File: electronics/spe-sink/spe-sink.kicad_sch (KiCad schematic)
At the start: 14 parts, among them J1 CONN_01X05_RA

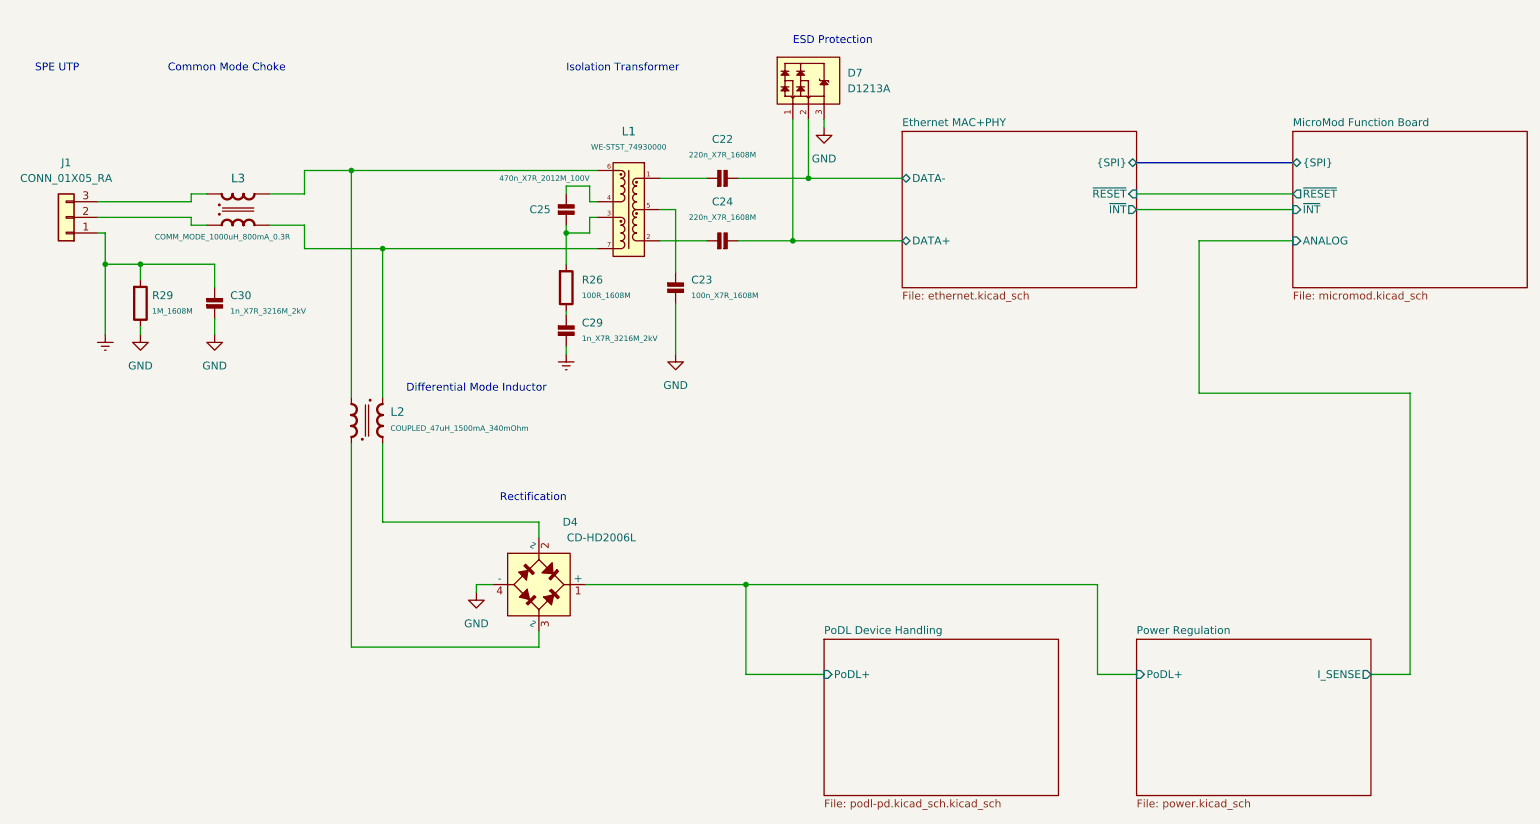
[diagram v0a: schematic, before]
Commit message: Random uncommitted KiCAD tweaks
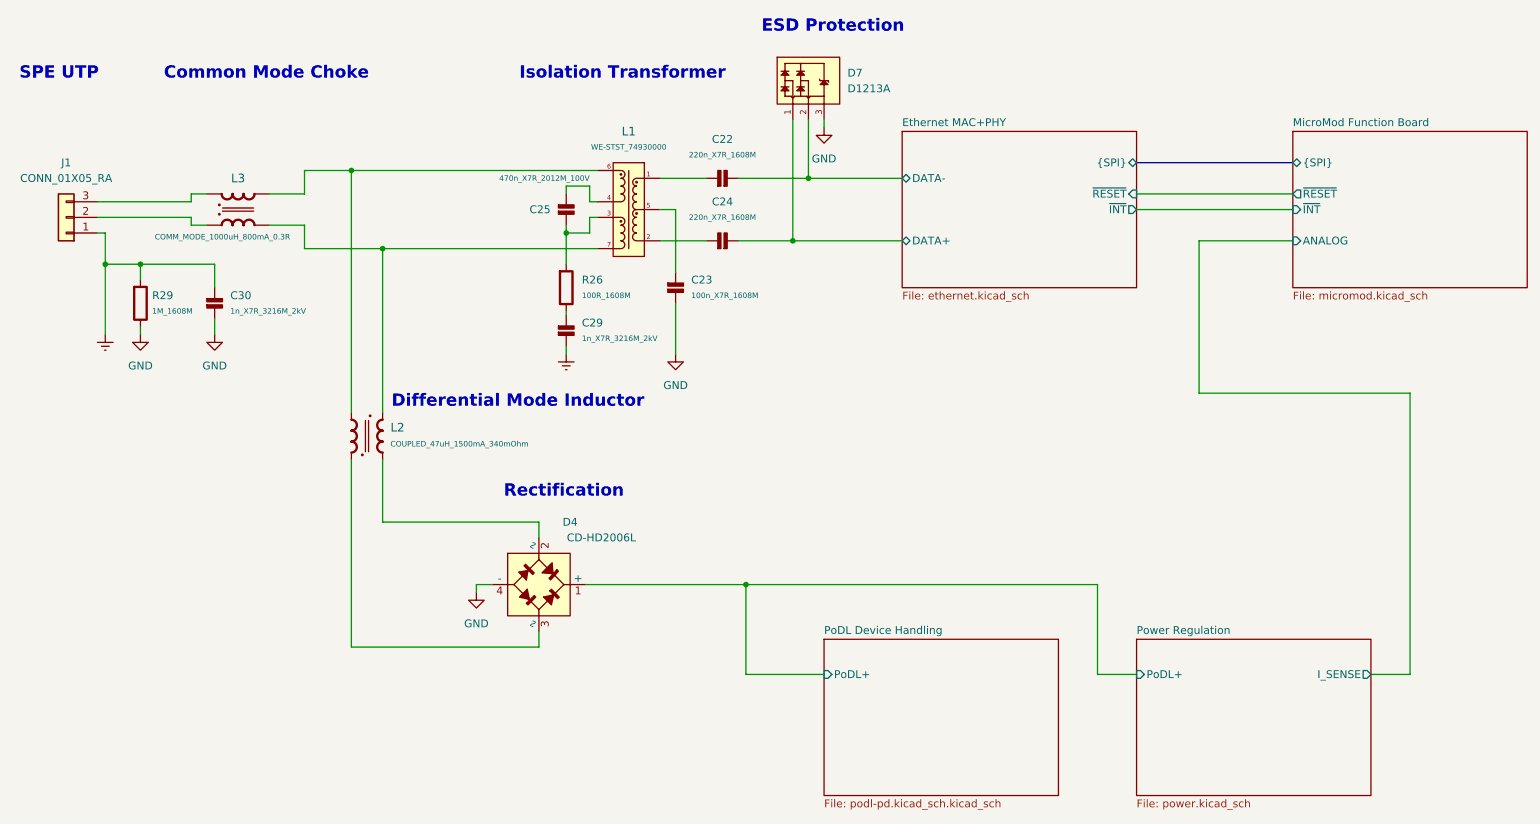
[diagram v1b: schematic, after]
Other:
- moved on the sheet: L2
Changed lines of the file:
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@@
     (comment 1 "Prototype Design")
   )
+  (bus_alias "I2C" (members "SDA" "SCL"))
   (bus_alias "SPI" (members "COPI" "CIPO" "CLK" "~{CS}"))
-  (bus_alias "I2C" (members "SDA" "SCL"))
   (junction (at 110.49 54.61) (diameter 0) (color 0 0 0 0)
   )
@@
     (stroke (width 0) (type default))
   )
-  (wire (pts (xy 80.645 57.15) (xy 80.645 81.28))
-    (stroke (width 0) (type default))
-  )
-  (wire (pts (xy 75.565 88.9) (xy 75.565 121.92))
+  (wire (pts (xy 80.645 57.15) (xy 80.645 83.82))
+    (stroke (width 0) (type default))
+  )
+  (wire (pts (xy 75.565 91.44) (xy 75.565 121.92))
     (stroke (width 0) (type default))
   )
@@
     (stroke (width 0) (type default))
   )
-  (wire (pts (xy 80.645 88.9) (xy 80.645 101.6))
+  (wire (pts (xy 80.645 91.44) (xy 80.645 101.6))
     (stroke (width 0) (type default))
   )
@@
     (stroke (width 0) (type default))
   )
-  (wire (pts (xy 75.565 44.45) (xy 75.565 81.28))
+  (wire (pts (xy 75.565 44.45) (xy 75.565 83.82))
     (stroke (width 0) (type default))
   )
@@
     (stroke (width 0) (type default))
   )
-  (text "Common Mode Choke" (at 45.72 28.575 0)
-    (effects (font (size 1.27 1.27)) (justify left bottom))
-  )
-  (text "Differential Mode Inductor" (at 107.315 80.645 0)
-    (effects (font (size 1.27 1.27)) (justify right bottom))
-  )
-  (text "ESD Protection" (at 147.32 24.13 0)
-    (effects (font (size 1.27 1.27)) (justify left bottom))
-  )
-  (text "Isolation Transformer" (at 110.49 28.575 0)
-    (effects (font (size 1.25 1.25)) (justify left bottom))
-  )
-  (text "SPE UTP" (at 24.13 28.575 0)
-    (effects (font (size 1.27 1.27)) (justify left bottom))
-  )
-  (text "Rectification" (at 99.695 98.425 0)
-    (effects (font (size 1.27 1.27)) (justify left bottom))
+  (text "Common Mode Choke" (at 45.085 29.845 0)
+    (effects (font (size 2 2) (thickness 0.4) bold) (justify left bottom))
+  )
+  (text "Differential Mode Inductor" (at 123.19 83.185 0)
+    (effects (font (size 2 2) (thickness 0.4) bold) (justify right bottom))
+  )
+  (text "ESD Protection" (at 142.24 22.225 0)
+    (effects (font (size 2 2) (thickness 0.4) bold) (justify left bottom))
+  )
+  (text "Isolation Transformer" (at 102.87 29.845 0)
+    (effects (font (size 2 2) (thickness 0.4) bold) (justify left bottom))
+  )
+  (text "SPE UTP" (at 21.59 29.845 0)
+    (effects (font (size 2 2) (thickness 0.4) bold) (justify left bottom))
+  )
+  (text "Rectification" (at 100.33 97.79 0)
+    (effects (font (size 2 2) (thickness 0.4) bold) (justify left bottom))
   )
   (symbol (lib_id "appli_resistor:1M_1608M") (at 41.275 62.23 0) (unit 1)
@@
     )
   )
-  (symbol (lib_id "appli_inductor:COUPLED_47uH_1500mA_340mOhm") (at 78.105 85.09 90) (unit 1)
+  (symbol (lib_id "appli_inductor:COUPLED_47uH_1500mA_340mOhm") (at 78.105 87.63 90) (unit 1)
     (in_bom yes) (on_board yes) (dnp no)
-    (property "Reference" "L2" (at 81.915 83.6929 90)
+    (property "Reference" "L2" (at 81.915 86.2329 90)
       (effects (font (size 1.397 1.397)) (justify right))
     )
-    (property "Value" "COUPLED_47uH_1500mA_340mOhm" (at 81.915 86.36 90)
+    (property "Value" "COUPLED_47uH_1500mA_340mOhm" (at 81.915 88.9 90)
       (effects (font (size 0.889 0.889)) (justify right))
     )
-    (property "Footprint" "Applidyne_Inductor:WE-MCRI-1040" (at 84.836 85.09 0)
-      (effects (font (size 0.508 0.508)) hide)
-    )
-    (property "Datasheet" "https://www.we-online.com/components/products/datasheet/7448991470.pdf" (at 85.471 85.09 0)
-      (effects (font (size 0.508 0.508)) hide)
-    )
-    (property "manf" "Würth Elektronik" (at 86.741 85.09 0)
-      (effects (font (size 0.508 0.508)) hide)
-    )
-    (property "manf#" "7448991470" (at 87.376 85.09 0)
-      (effects (font (size 0.508 0.508)) hide)
-    )
-    (property "Supplier" "Digikey" (at 88.011 85.09 0)
-      (effects (font (size 0.508 0.508)) hide)
-    )
-    (property "Supplier Part No" "732-13378-1-ND" (at 88.646 85.09 0)
-      (effects (font (size 0.508 0.508)) hide)
-    )
-    (property "Supplier URL" "https://www.digikey.com.au/en/products/detail/w%C3%BCrth-elektronik/7448991470/9857425" (at 89.281 85.09 0)
-      (effects (font (size 0.508 0.508)) hide)
-    )
-    (property "Supplier Price" "5.60" (at 89.916 85.09 0)
-      (effects (font (size 0.508 0.508)) hide)
-    )
-    (property "Supplier Price Break" "1" (at 90.551 85.09 0)
-      (effects (font (size 0.508 0.508)) hide)
-    )
+    (property "Footprint" "Applidyne_Inductor:WE-MCRI-1040" (at 84.836 87.63 0)
+      (effects (font (size 0.508 0.508)) hide)
+    )
+    (property "Datasheet" "https://www.we-online.com/components/products/datasheet/7448991470.pdf" (at 85.471 87.63 0)
+      (effects (font (size 0.508 0.508)) hide)
+    )
+    (property "manf" "Würth Elektronik" (at 86.741 87.63 0)
+      (effects (font (size 0.508 0.508)) hide)
+    )
+    (property "manf#" "7448991470" (at 87.376 87.63 0)
+      (effects (font (size 0.508 0.508)) hide)
+    )
+    (property "Supplier" "Digikey" (at 88.011 87.63 0)
+      (effects (font (size 0.508 0.508)) hide)
+    )
+    (property "Supplier Part No" "732-13378-1-ND" (at 88.646 87.63 0)
+      (effects (font (size 0.508 0.508)) hide)
+    )
+    (property "Supplier URL" "https://www.digikey.com.au/en/products/detail/w%C3%BCrth-elektronik/7448991470/9857425" (at 89.281 87.63 0)
+      (effects (font (size 0.508 0.508)) hide)
+    )
+    (property "Supplier Price" "5.60" (at 89.916 87.63 0)
+      (effects (font (size 0.508 0.508)) hide)
+    )
+    (property "Supplier Price Break" "1" (at 90.551 87.63 0)
+      (effects (font (size 0.508 0.508)) hide)
+    )
